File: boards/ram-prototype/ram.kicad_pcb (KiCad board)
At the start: 4 copper layers, 221 x 106 mm, 611 parts, among them J1 PinHeader_1x24_P2.54mm_Vertic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, J2 PinHeader_1x04_P2.54mm_Vertic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, J3 PinHeader_1x16_P2.54mm_Vertic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, J4 PinHeader_1x14_P2.54mm_Vertic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, U1 DSBGA\-5_NumericPads, U10 DSBGA\-5_NumericPads, U100 DSBGA\-5_NumericPads, U101 DSBGA\-5_NumericPads, U102 DSBGA\-5_NumericPads, U103 DSBGA\-5_NumericPads, U104 DSBGA\-5_NumericPads, U105 DSBGA\-5_NumericPads, U106 DSBGA\-5_NumericPads, U107 DSBGA\-5_NumericPads, U108 DSBGA\-5_NumericPads, U109 DSBGA\-5_NumericPads, U11 DSBGA\-5_NumericPads, U110 DSBGA\-5_NumericPads, U111 DSBGA\-5_NumericPads, U112 DSBGA\-5_NumericPads, U113 DSBGA\-5_NumericPads, U114 DSBGA\-5_NumericPads, U115 DSBGA\-5_NumericPads, U116 DSBGA\-5_NumericPads, U117 DSBGA\-5_NumericPads, U118 DSBGA\-5_NumericPads, U119 DSBGA\-5_NumericPads, U12 DSBGA\-5_NumericPads, U120 DSBGA\-5_NumericPads, U121 DSBGA\-5_NumericPads, U122 DSBGA\-5_NumericPads, U123 DSBGA\-5_NumericPads, U124 DSBGA\-5_NumericPads, U125 DSBGA\-5_NumericPads, U126 DSBGA\-5_NumericPads, U127 DSBGA\-5_NumericPads, U128 DSBGA\-5_NumericPads, U129 DSBGA\-5_NumericPads, U13 DSBGA\-5_NumericPads, U130 DSBGA\-5_NumericPads, U131 DSBGA\-5_NumericPads, U132 DSBGA\-5_NumericPads, U133 DSBGA\-5_NumericPads, U134 DSBGA\-5_NumericPads, U135 DSBGA\-5_NumericPads, U136 DSBGA\-5_NumericPads, U137 DSBGA\-5_NumericPads, U138 DSBGA\-5_NumericPads, U139 DSBGA\-5_NumericPads, U14 DSBGA\-5_NumericPads, U140 DSBGA\-5_NumericPads, U141 DSBGA\-5_NumericPads, U142 DSBGA\-5_NumericPads, U143 DSBGA\-5_NumericPads, U144 DSBGA\-5_NumericPads, U145 DSBGA\-5_NumericPads, U146 DSBGA\-5_NumericPads, U147 DSBGA\-5_NumericPads, U148 DSBGA\-5_NumericPads, U149 DSBGA\-5_NumericPads, U15 DSBGA\-5_NumericPads, U150 DSBGA\-5_NumericPads, U151 DSBGA\-5_NumericPads, U152 DSBGA\-5_NumericPads, U153 DSBGA\-5_NumericPads, U154 DSBGA\-5_NumericPads, U155 DSBGA\-5_NumericPads, U156 DSBGA\-5_NumericPads, U157 DSBGA\-5_NumericPads, U158 DSBGA\-5_NumericPads, U159 DSBGA\-5_NumericPads, U16 DSBGA\-5_NumericPads, U160 DSBGA\-5_NumericPads, U161 DSBGA\-5_NumericPads, U162 DSBGA\-5_NumericPads, U163 DSBGA\-5_NumericPads, U164 DSBGA\-5_NumericPads, U165 DSBGA\-5_NumericPads, U166 DSBGA\-5_NumericPads, U167 DSBGA\-5_NumericPads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

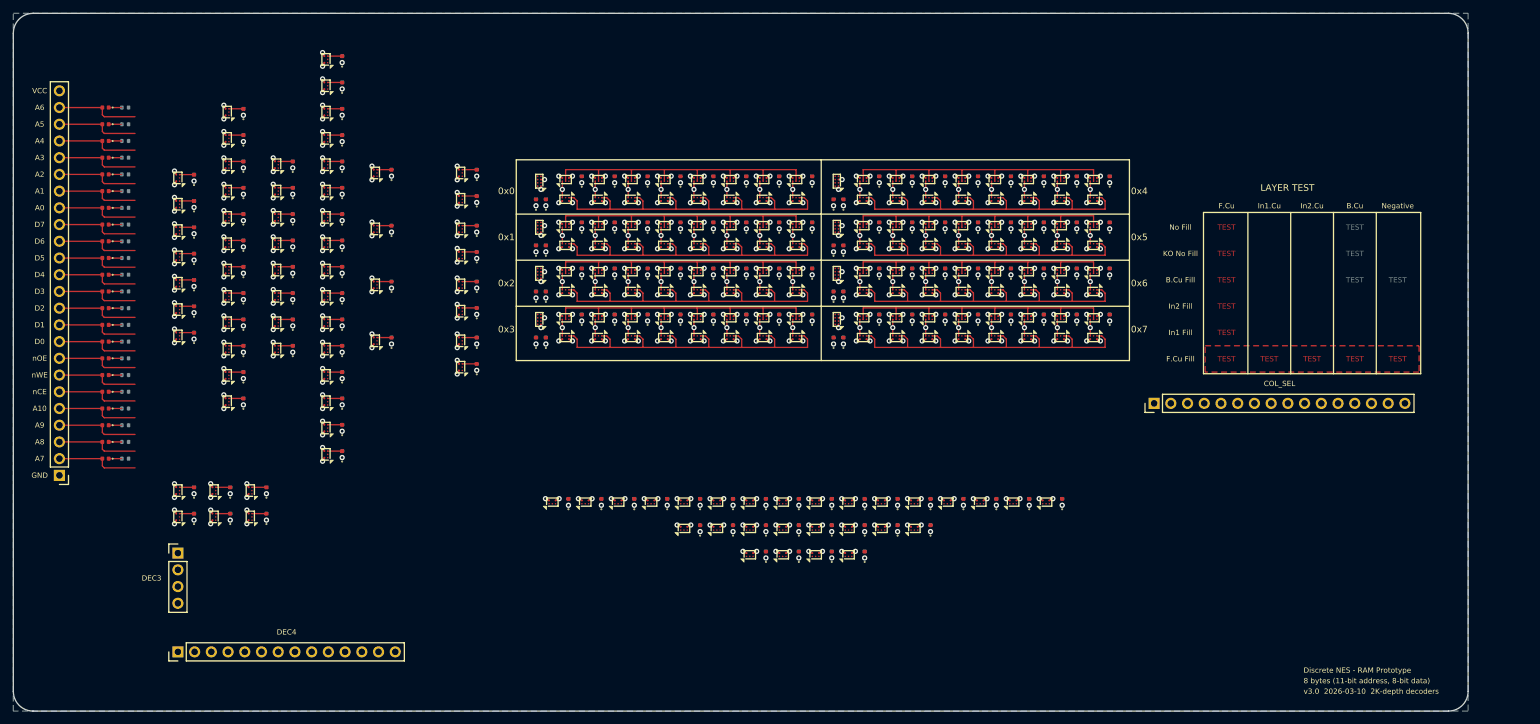
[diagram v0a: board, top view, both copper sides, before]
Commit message: Fix a bunch of issues
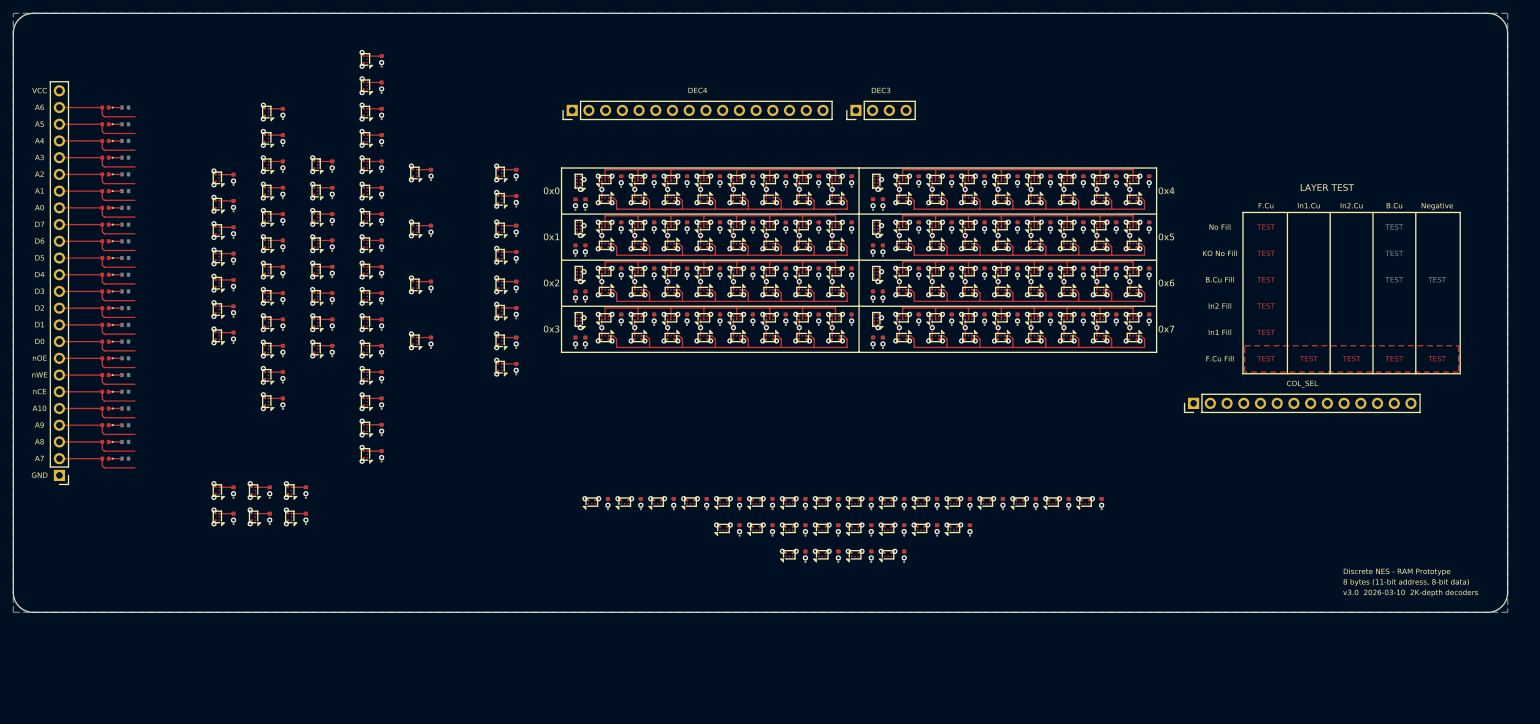
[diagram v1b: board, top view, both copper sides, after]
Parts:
- J3: value PinHeader_1x16_P2.54mm_Vertical -> PinHeader_1x14_P2.54mm_Vertical; footprint Connector_PinHeader_2.54mm:PinHeader_1x16_P2.54mm_Vertical -> Connector_PinHeader_2.54mm:PinHeader_1x14_P2.54mm_Vertical
- J4: value PinHeader_1x14_P2.54mm_Vertical -> PinHeader_1x16_P2.54mm_Vertical; footprint Connector_PinHeader_2.54mm:PinHeader_1x14_P2.54mm_Vertical -> Connector_PinHeader_2.54mm:PinHeader_1x16_P2.54mm_Vertical
- moved J2 123.0 mm to (141.0, 27.8), turned to 90 degrees
- moved J4 101.8 mm to (97.9, 27.8)
- moved D70 6.00 mm to (133.3, 95.2)
- moved D75 6.00 mm to (128.3, 91.2)
- moved D76 6.00 mm to (133.3, 91.2)
- moved D87 6.00 mm to (128.3, 87.2)
- moved D88 6.00 mm to (133.3, 87.2)
- moved R70 6.00 mm to (133.3, 95.2)
- moved R75 6.00 mm to (128.3, 91.2)
- moved R76 6.00 mm to (133.3, 91.2)
- moved R87 6.00 mm to (128.3, 87.2)
- moved R88 6.00 mm to (133.3, 87.2)
- moved D100 6.00 mm to (89.4, 54.2)
- moved D101 6.00 mm to (89.4, 62.8)
- moved D102 6.00 mm to (89.4, 41.2)
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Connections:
- D23 pad 2: /Address Decoder/nA0 -> /Address Decoder/nA6
- D24 pad 2: /Address Decoder/nA1 -> /Address Decoder/nA5
- D25 pad 2: /Address Decoder/nA2 -> /Address Decoder/nA4
- D27 pad 2: /Address Decoder/nA4 -> /Address Decoder/nA2
- D28 pad 2: /Address Decoder/nA5 -> /Address Decoder/nA1
- D29 pad 2: /Address Decoder/nA6 -> /Address Decoder/nA0
- J3 pad 1: /DEC4_1 -> /COL_SEL_2
- J3 pad 10: /DEC4_10 -> /COL_SEL_11
- J3 pad 11: /DEC4_11 -> /COL_SEL_12
- J3 pad 12: /DEC4_12 -> /COL_SEL_13
- J3 pad 13: /DEC4_13 -> /COL_SEL_14
- J3 pad 14: /DEC4_14 -> /COL_SEL_15
- J3 pad 2: /DEC4_2 -> /COL_SEL_3
- J3 pad 3: /DEC4_3 -> /COL_SEL_4
- J3 pad 4: /DEC4_4 -> /COL_SEL_5
- J3 pad 5: /DEC4_5 -> /COL_SEL_6
- J3 pad 6: /DEC4_6 -> /COL_SEL_7
- J3 pad 7: /DEC4_7 -> /COL_SEL_8
- J3 pad 8: /DEC4_8 -> /COL_SEL_9
- J3 pad 9: /DEC4_9 -> /COL_SEL_10
- J4 pad 1: /COL_SEL_2 -> /DEC4_1
- J4 pad 10: /COL_SEL_11 -> /DEC4_10
- J4 pad 11: /COL_SEL_12 -> /DEC4_11
- J4 pad 12: /COL_SEL_13 -> /DEC4_12
- J4 pad 13: /COL_SEL_14 -> /DEC4_13
- J4 pad 14: /COL_SEL_15 -> /DEC4_14
- J4 pad 2: /COL_SEL_3 -> /DEC4_2
- J4 pad 3: /COL_SEL_4 -> /DEC4_3
- J4 pad 4: /COL_SEL_5 -> /DEC4_4
- J4 pad 5: /COL_SEL_6 -> /DEC4_5
- J4 pad 6: /COL_SEL_7 -> /DEC4_6
- J4 pad 7: /COL_SEL_8 -> /DEC4_7
- J4 pad 8: /COL_SEL_9 -> /DEC4_8
- J4 pad 9: /COL_SEL_10 -> /DEC4_9
- U1 pad 2: /Address Decoder/A0 -> /Address Decoder/A6
- U1 pad 4: /Address Decoder/nA0 -> /Address Decoder/nA6
- U2 pad 2: /Address Decoder/A1 -> /Address Decoder/A5
- U2 pad 4: /Address Decoder/nA1 -> /Address Decoder/nA5
- U3 pad 2: /Address Decoder/A2 -> /Address Decoder/A4
- U3 pad 4: /Address Decoder/nA2 -> /Address Decoder/nA4
- U5 pad 2: /Address Decoder/A4 -> /Address Decoder/A2
- U5 pad 4: /Address Decoder/nA4 -> /Address Decoder/nA2
- U6 pad 2: /Address Decoder/A5 -> /Address Decoder/A1
- U6 pad 4: /Address Decoder/nA5 -> /Address Decoder/nA1
- U7 pad 2: /Address Decoder/A6 -> /Address Decoder/A0
- U7 pad 4: /Address Decoder/nA6 -> /Address Decoder/nA0
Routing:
- added copper zone on In1.Cu, net GND
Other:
- board size 221 x 106 mm -> 227 x 91 mm

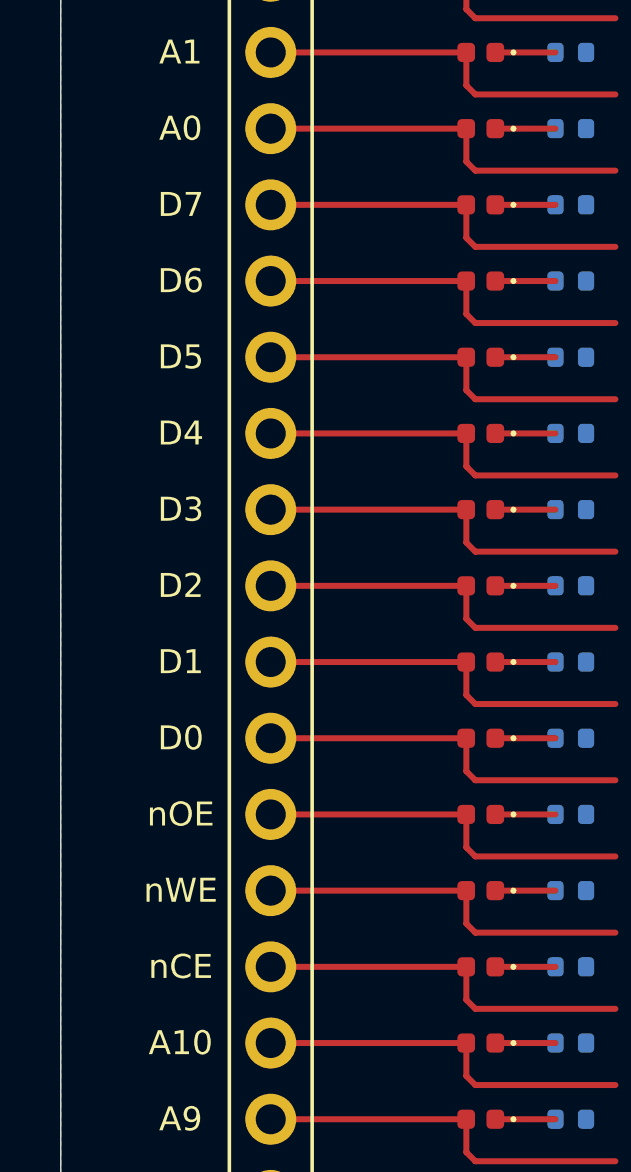
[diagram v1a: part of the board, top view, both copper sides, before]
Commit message: Fix more issues
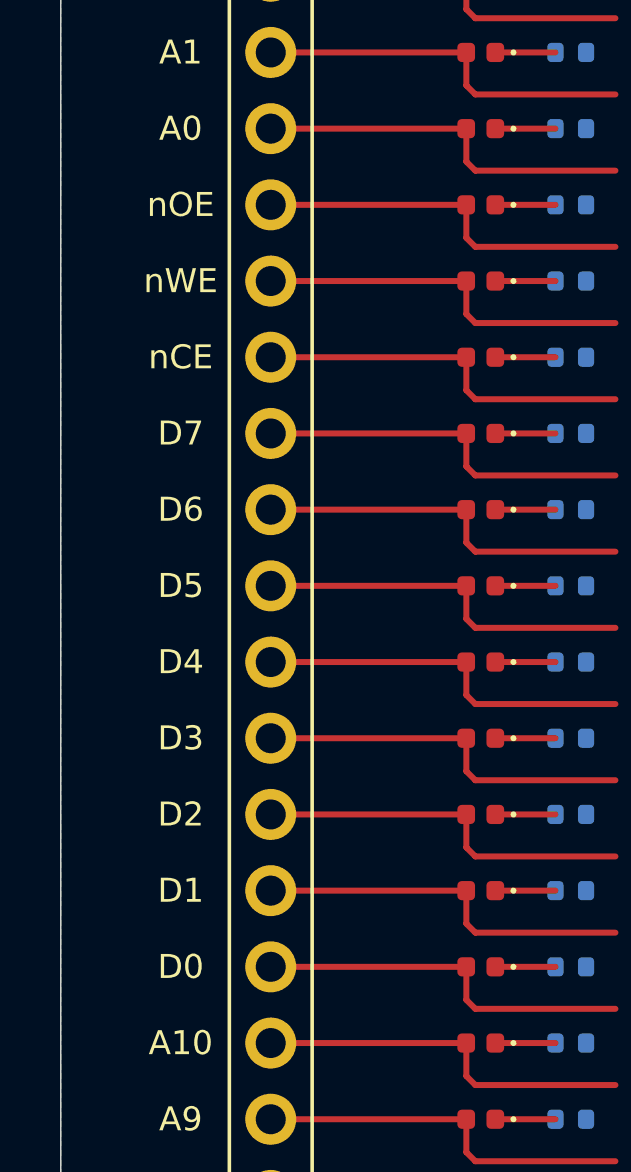
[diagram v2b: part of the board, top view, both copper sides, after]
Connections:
- D10 pad 2: /D5 -> /nCE
- D11 pad 2: /D4 -> /D7
- D12 pad 2: /D3 -> /D6
- D13 pad 2: /D2 -> /D5
- D14 pad 2: /D1 -> /D4
- D15 pad 2: /D0 -> /D3
- D16 pad 2: /nOE -> /D2
- D17 pad 2: /nWE -> /D1
- D18 pad 2: /nCE -> /D0
- D8 pad 2: /D7 -> /nOE
- D9 pad 2: /D6 -> /nWE
- J1 pad 10: /D1 -> /D4
- J1 pad 11: /D2 -> /D5
- J1 pad 12: /D3 -> /D6
- J1 pad 13: /D4 -> /D7
- J1 pad 14: /D5 -> /nCE
- J1 pad 15: /D6 -> /nWE
- J1 pad 16: /D7 -> /nOE
- J1 pad 6: /nCE -> /D0
- J1 pad 7: /nWE -> /D1
- J1 pad 8: /nOE -> /D2
- J1 pad 9: /D0 -> /D3
